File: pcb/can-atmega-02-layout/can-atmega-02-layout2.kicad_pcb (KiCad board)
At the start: 2 copper layers, 114 x 98 mm, 168 parts, among them J1 Screw_Terminal_01x05, J3 Conn_02x03_Odd_Even, J4 Connector_female, U1 LM1117-5.0, U2 TJA1051T, U3 MCP2515-xSO, U4 ATmega328P-A, X1 16MHz, X2 16MHz

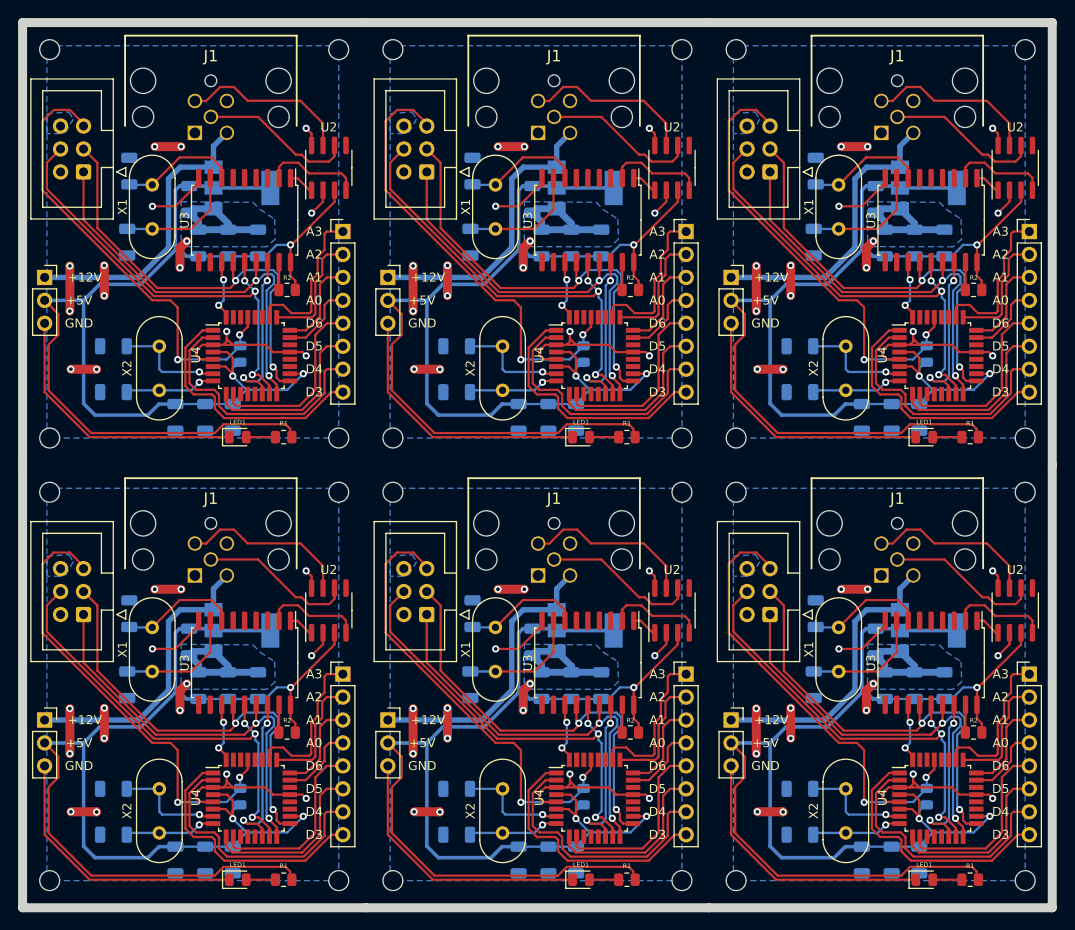
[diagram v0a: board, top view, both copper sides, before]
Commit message: temp-calibrate
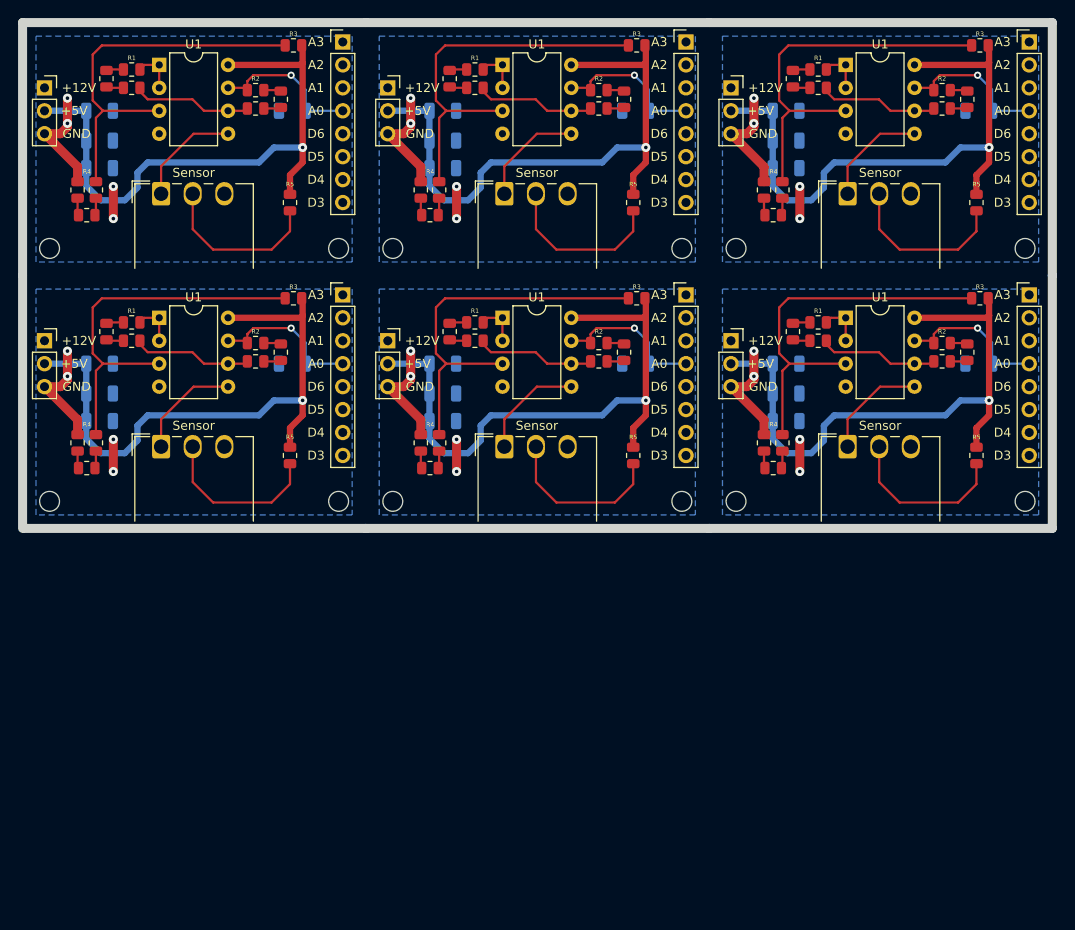
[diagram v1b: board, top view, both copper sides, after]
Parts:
- removed the C1 at (107.9, 33.1)
- removed the C1 at (69.9, 82.1)
- removed the C1 at (69.9, 33.1)
- removed the C1 at (31.9, 82.1)
- removed the C1 at (107.9, 82.1)
- removed the C1 at (31.9, 33.1)
- removed C10 (x6), C11 (x6), C5 (x6), C6 (x6): 22PF, Capacitor_SMD:C_1206_3216Metric
- removed the C2 at (71.0, 37.9)
- removed the C2 at (33.0, 37.9)
- removed the C2 at (109.0, 37.9)
- removed the C2 at (71.0, 86.9)
- removed the C2 at (109.0, 86.9)
- removed the C2 at (33.0, 86.9)
- removed the C3 at (112.3, 37.9)
- removed the C3 at (36.3, 37.9)
- removed the C3 at (112.3, 86.9)
- removed the C3 at (74.3, 37.9)
- removed the C3 at (36.3, 86.9)
- removed the C3 at (74.3, 86.9)
- removed the C4 at (77.6, 37.9)
- removed the C4 at (39.6, 37.9)
- removed the C4 at (39.6, 86.9)
- removed the C4 at (115.6, 86.9)
- removed the C4 at (115.6, 37.9)
- removed the C4 at (77.6, 86.9)
- removed C7 (x6), C9 (x6): 0.1uF, Capacitor_SMD:C_1206_3216Metric
- removed C8 (x6): 10uF/16V, Capacitor_SMD:C_1206_3216Metric
- removed the J1 at (32.6, 74.7)
- removed the J1 at (32.6, 25.7)
- removed the J1 at (70.6, 25.7)
- removed the J1 at (70.6, 74.7)
- removed the J1 at (108.6, 74.7)
- removed the J1 at (108.6, 25.7)
- removed J3 (x6): Conn_02x03_Odd_Even, Connector_IDC:IDC-Header_2x03_P2.54mm_Vertical
- removed J4 (x6): Connector_female, CAN_ATmega:Connector_female
- removed LED1 (x6): Green, LED_SMD:LED_0805_2012Metric
- removed R1 (x6): 1K, Resistor_SMD:R_0805_2012Metric
- removed R2 (x6): 10K, Resistor_SMD:R_0805_2012Metric
- removed the R3 at (75.6, 99.2)
- removed the R3 at (75.6, 50.2)
- removed the R3 at (37.6, 50.2)
- removed the R3 at (37.6, 99.2)
- removed the R3 at (113.6, 99.2)
- removed the R3 at (113.6, 50.2)
- removed the REF** at (48.5, 16.5)
- removed the REF** at (54.5, 59.5)
- removed the REF** at (54.5, 65.5)
- removed the REF** at (86.5, 108.5)
- removed the REF** at (92.5, 65.5)
- removed the REF** at (16.5, 108.5)
- removed the REF** at (16.5, 65.5)
- removed the REF** at (86.5, 16.5)
- removed the REF** at (92.5, 16.5)
- removed the REF** at (48.5, 65.5)
- removed the REF** at (124.5, 16.5)
- removed the REF** at (124.5, 65.5)
- removed the REF** at (124.5, 59.5)
- removed the REF** at (92.5, 59.5)
- removed the REF** at (48.5, 108.5)
- removed the REF** at (124.5, 108.5)
- removed the REF** at (48.5, 59.5)
- removed the REF** at (54.5, 16.5)
- removed the REF** at (92.5, 108.5)
- removed the REF** at (86.5, 65.5)
- removed the REF** at (16.5, 59.5)
- removed the REF** at (16.5, 16.5)
- removed the REF** at (86.5, 59.5)
- removed the REF** at (54.5, 108.5)
- removed the U1 at (75.8, 80.8)
- removed the U1 at (37.8, 31.8)
- removed the U1 at (113.8, 80.8)
- removed the U1 at (75.8, 31.8)
- removed the U1 at (113.8, 31.8)
- removed the U1 at (37.8, 80.8)
- removed U2 (x6): TJA1051T, Package_SO:SOIC-8_3.9x4.9mm_P1.27mm
- removed U3 (x6): MCP2515-xSO, Package_SO:SOIC-18W_7.5x11.6mm_P1.27mm
- removed U4 (x6): ATmega328P-A, Package_QFP:TQFP-32_7x7mm_P0.8mm
- removed X1 (x6), X2 (x6): 16MHz, Crystal:Crystal_HC49-4H_Vertical
- added C1: 100nF, Capacitor_SMD:C_1206_3216Metric, B.Cu at (22.0, 23.3)
- added C1: 100nF, Capacitor_SMD:C_1206_3216Metric, B.Cu at (22.0, 51.3)
- added C1: 100nF, Capacitor_SMD:C_1206_3216Metric, B.Cu at (98.0, 23.3)
- added C1: 100nF, Capacitor_SMD:C_1206_3216Metric, B.Cu at (60.0, 51.3)
- added C1: 100nF, Capacitor_SMD:C_1206_3216Metric, B.Cu at (60.0, 23.3)
- added C1: 100nF, Capacitor_SMD:C_1206_3216Metric, B.Cu at (98.0, 51.3)
- added C2: 100nF, Capacitor_SMD:C_1206_3216Metric, B.Cu at (98.0, 54.6)
- added C2: 100nF, Capacitor_SMD:C_1206_3216Metric, B.Cu at (98.0, 26.6)
- added C2: 100nF, Capacitor_SMD:C_1206_3216Metric, B.Cu at (22.0, 54.6)
- added C2: 100nF, Capacitor_SMD:C_1206_3216Metric, B.Cu at (60.0, 26.6)
- added C2: 100nF, Capacitor_SMD:C_1206_3216Metric, B.Cu at (22.0, 26.6)
- added C2: 100nF, Capacitor_SMD:C_1206_3216Metric, B.Cu at (60.0, 54.6)
- added C3: 10uF/16V, Capacitor_SMD:C_1206_3216Metric, B.Cu at (60.0, 57.6)
- added C3: 10uF/16V, Capacitor_SMD:C_1206_3216Metric, B.Cu at (22.0, 57.6)
- added C3: 10uF/16V, Capacitor_SMD:C_1206_3216Metric, B.Cu at (60.0, 29.6)
- added C3: 10uF/16V, Capacitor_SMD:C_1206_3216Metric, B.Cu at (98.0, 29.6)
- added C3: 10uF/16V, Capacitor_SMD:C_1206_3216Metric, B.Cu at (22.0, 29.6)
- added C3: 10uF/16V, Capacitor_SMD:C_1206_3216Metric, B.Cu at (98.0, 57.6)
- added C4: 100nF, Capacitor_SMD:C_1206_3216Metric, B.Cu at (119.4, 51.3)
- added C4: 100nF, Capacitor_SMD:C_1206_3216Metric, B.Cu at (81.4, 51.3)
- added C4: 100nF, Capacitor_SMD:C_1206_3216Metric, B.Cu at (81.4, 23.3)
- added C4: 100nF, Capacitor_SMD:C_1206_3216Metric, B.Cu at (43.4, 51.3)
- added C4: 100nF, Capacitor_SMD:C_1206_3216Metric, B.Cu at (119.4, 23.3)
- added C4: 100nF, Capacitor_SMD:C_1206_3216Metric, B.Cu at (43.4, 23.3)
- added J1: Connector_male, CAN_ATmega:Connector_male, F.Cu at (107.2, 23.3)
- added J1: Connector_male, CAN_ATmega:Connector_male, F.Cu at (31.2, 51.3)
- added J1: Connector_male, CAN_ATmega:Connector_male, F.Cu at (69.2, 23.3)
- added J1: Connector_male, CAN_ATmega:Connector_male, F.Cu at (107.2, 51.3)
- added J1: Connector_male, CAN_ATmega:Connector_male, F.Cu at (69.2, 51.3)
- added J1: Connector_male, CAN_ATmega:Connector_male, F.Cu at (31.2, 23.3)
- added J2: Screw_Terminal_01x03, Connector_Wago:Wago_734-163_1x03_P3.50mm_Horizontal, F.Cu at (66.8, 32.5)
- added J2: Screw_Terminal_01x03, Connector_Wago:Wago_734-163_1x03_P3.50mm_Horizontal, F.Cu at (28.8, 32.5)
- added J2: Screw_Terminal_01x03, Connector_Wago:Wago_734-163_1x03_P3.50mm_Horizontal, F.Cu at (104.8, 60.5)
- added J2: Screw_Terminal_01x03, Connector_Wago:Wago_734-163_1x03_P3.50mm_Horizontal, F.Cu at (66.8, 60.5)
- added J2: Screw_Terminal_01x03, Connector_Wago:Wago_734-163_1x03_P3.50mm_Horizontal, F.Cu at (104.8, 32.5)
- added J2: Screw_Terminal_01x03, Connector_Wago:Wago_734-163_1x03_P3.50mm_Horizontal, F.Cu at (28.8, 60.5)
- added R1_1: 1.3k, Resistor_SMD:R_0805_2012Metric, F.Cu at (101.6, 18.7)
- added R1_1: 1.3k, Resistor_SMD:R_0805_2012Metric, F.Cu at (101.6, 46.7)
- added R1_1: 1.3k, Resistor_SMD:R_0805_2012Metric, F.Cu at (63.6, 46.7)
- added R1_1: 1.3k, Resistor_SMD:R_0805_2012Metric, F.Cu at (25.6, 46.7)
- added R1_1: 1.3k, Resistor_SMD:R_0805_2012Metric, F.Cu at (25.6, 18.7)
- added R1_1: 1.3k, Resistor_SMD:R_0805_2012Metric, F.Cu at (63.6, 18.7)
- added R1_2: 2k, Resistor_SMD:R_0805_2012Metric, F.Cu at (60.8, 47.7)
- added R1_2: 2k, Resistor_SMD:R_0805_2012Metric, F.Cu at (22.8, 47.7)
- added R1_2: 2k, Resistor_SMD:R_0805_2012Metric, F.Cu at (22.8, 19.7)
- added R1_2: 2k, Resistor_SMD:R_0805_2012Metric, F.Cu at (98.8, 47.7)
- added R1_2: 2k, Resistor_SMD:R_0805_2012Metric, F.Cu at (98.8, 19.7)
- added R1_2: 2k, Resistor_SMD:R_0805_2012Metric, F.Cu at (60.8, 19.7)
- added R1_3: 10k, Resistor_SMD:R_0805_2012Metric, F.Cu at (63.6, 20.7)
- added R1_3: 10k, Resistor_SMD:R_0805_2012Metric, F.Cu at (101.6, 48.7)
- added R1_3: 10k, Resistor_SMD:R_0805_2012Metric, F.Cu at (25.6, 20.7)
- added R1_3: 10k, Resistor_SMD:R_0805_2012Metric, F.Cu at (101.6, 20.7)
- added R1_3: 10k, Resistor_SMD:R_0805_2012Metric, F.Cu at (63.6, 48.7)
- added R1_3: 10k, Resistor_SMD:R_0805_2012Metric, F.Cu at (25.6, 48.7)
- added R2_1: 330, Resistor_SMD:R_0805_2012Metric, F.Cu at (115.3, 23.0)
- added R2_1: 330, Resistor_SMD:R_0805_2012Metric, F.Cu at (77.3, 23.0)
- added R2_1: 330, Resistor_SMD:R_0805_2012Metric, F.Cu at (39.3, 23.0)
- added R2_1: 330, Resistor_SMD:R_0805_2012Metric, F.Cu at (115.3, 51.0)
- added R2_1: 330, Resistor_SMD:R_0805_2012Metric, F.Cu at (39.3, 51.0)
- added R2_1: 330, Resistor_SMD:R_0805_2012Metric, F.Cu at (77.3, 51.0)
- added R2_2: 1.3k, Resistor_SMD:R_0805_2012Metric, F.Cu at (42.1, 22.0)
- added R2_2: 1.3k, Resistor_SMD:R_0805_2012Metric, F.Cu at (80.1, 22.0)
- added R2_2: 1.3k, Resistor_SMD:R_0805_2012Metric, F.Cu at (118.1, 22.0)
- added R2_2: 1.3k, Resistor_SMD:R_0805_2012Metric, F.Cu at (80.1, 50.0)
- added R2_2: 1.3k, Resistor_SMD:R_0805_2012Metric, F.Cu at (118.1, 50.0)
- added R2_2: 1.3k, Resistor_SMD:R_0805_2012Metric, F.Cu at (42.1, 50.0)
- added R2_3: 110k, Resistor_SMD:R_0805_2012Metric, F.Cu at (77.3, 21.0)
- added R2_3: 110k, Resistor_SMD:R_0805_2012Metric, F.Cu at (39.3, 21.0)
- added R2_3: 110k, Resistor_SMD:R_0805_2012Metric, F.Cu at (39.3, 49.0)
- added R2_3: 110k, Resistor_SMD:R_0805_2012Metric, F.Cu at (77.3, 49.0)
- added R2_3: 110k, Resistor_SMD:R_0805_2012Metric, F.Cu at (115.3, 21.0)
- added R2_3: 110k, Resistor_SMD:R_0805_2012Metric, F.Cu at (115.3, 49.0)
- added R3: 20k, Resistor_SMD:R_0805_2012Metric, F.Cu at (81.5, 44.0)
- added R3: 20k, Resistor_SMD:R_0805_2012Metric, F.Cu at (119.5, 16.0)
- added R3: 20k, Resistor_SMD:R_0805_2012Metric, F.Cu at (43.5, 16.0)
- added R3: 20k, Resistor_SMD:R_0805_2012Metric, F.Cu at (81.5, 16.0)
- added R3: 20k, Resistor_SMD:R_0805_2012Metric, F.Cu at (119.5, 44.0)
- added R3: 20k, Resistor_SMD:R_0805_2012Metric, F.Cu at (43.5, 44.0)
- added R4_1: 2k, Resistor_SMD:R_0805_2012Metric, F.Cu at (57.6, 32.0)
- added R4_1: 2k, Resistor_SMD:R_0805_2012Metric, F.Cu at (19.6, 32.0)
- added R4_1: 2k, Resistor_SMD:R_0805_2012Metric, F.Cu at (95.6, 60.0)
- added R4_1: 2k, Resistor_SMD:R_0805_2012Metric, F.Cu at (57.6, 60.0)
- added R4_1: 2k, Resistor_SMD:R_0805_2012Metric, F.Cu at (95.6, 32.0)
- added R4_1: 2k, Resistor_SMD:R_0805_2012Metric, F.Cu at (19.6, 60.0)
- added R4_2: 2.4k, Resistor_SMD:R_0805_2012Metric, F.Cu at (20.6, 34.8)
- added R4_2: 2.4k, Resistor_SMD:R_0805_2012Metric, F.Cu at (96.6, 62.8)
- added R4_2: 2.4k, Resistor_SMD:R_0805_2012Metric, F.Cu at (58.6, 34.8)
- added R4_2: 2.4k, Resistor_SMD:R_0805_2012Metric, F.Cu at (20.6, 62.8)
- added R4_2: 2.4k, Resistor_SMD:R_0805_2012Metric, F.Cu at (58.6, 62.8)
- added R4_2: 2.4k, Resistor_SMD:R_0805_2012Metric, F.Cu at (96.6, 34.8)
- added R4_3: 20k, Resistor_SMD:R_0805_2012Metric, F.Cu at (97.6, 32.0)
- added R4_3: 20k, Resistor_SMD:R_0805_2012Metric, F.Cu at (21.6, 60.0)
- added R4_3: 20k, Resistor_SMD:R_0805_2012Metric, F.Cu at (59.6, 32.0)
- added R4_3: 20k, Resistor_SMD:R_0805_2012Metric, F.Cu at (21.6, 32.0)
- added R4_3: 20k, Resistor_SMD:R_0805_2012Metric, F.Cu at (97.6, 60.0)
- added R4_3: 20k, Resistor_SMD:R_0805_2012Metric, F.Cu at (59.6, 60.0)
- added R5: 1k, Resistor_SMD:R_0805_2012Metric, F.Cu at (43.1, 33.4)
- added R5: 1k, Resistor_SMD:R_0805_2012Metric, F.Cu at (119.1, 61.4)
- added R5: 1k, Resistor_SMD:R_0805_2012Metric, F.Cu at (119.1, 33.4)
- added R5: 1k, Resistor_SMD:R_0805_2012Metric, F.Cu at (81.1, 33.4)
- added R5: 1k, Resistor_SMD:R_0805_2012Metric, F.Cu at (43.1, 61.4)
- added R5: 1k, Resistor_SMD:R_0805_2012Metric, F.Cu at (81.1, 61.4)
- added REF**: MountingHole_2.2mm_M2, MountingHole:MountingHole_2.2mm_M2, F.Cu at (92.5, 66.5)
- added REF**: MountingHole_2.2mm_M2, MountingHole:MountingHole_2.2mm_M2, F.Cu at (124.5, 38.5)
- added REF**: MountingHole_2.2mm_M2, MountingHole:MountingHole_2.2mm_M2, F.Cu at (54.5, 66.5)
- added REF**: MountingHole_2.2mm_M2, MountingHole:MountingHole_2.2mm_M2, F.Cu at (92.5, 38.5)
- added REF**: MountingHole_2.2mm_M2, MountingHole:MountingHole_2.2mm_M2, F.Cu at (16.5, 66.5)
- added REF**: MountingHole_2.2mm_M2, MountingHole:MountingHole_2.2mm_M2, F.Cu at (54.5, 38.5)
- added REF**: MountingHole_2.2mm_M2, MountingHole:MountingHole_2.2mm_M2, F.Cu at (48.5, 38.5)
- added REF**: MountingHole_2.2mm_M2, MountingHole:MountingHole_2.2mm_M2, F.Cu at (86.5, 38.5)
- added REF**: MountingHole_2.2mm_M2, MountingHole:MountingHole_2.2mm_M2, F.Cu at (86.5, 66.5)
- added REF**: MountingHole_2.2mm_M2, MountingHole:MountingHole_2.2mm_M2, F.Cu at (16.5, 38.5)
- added REF**: MountingHole_2.2mm_M2, MountingHole:MountingHole_2.2mm_M2, F.Cu at (124.5, 66.5)
- added REF**: MountingHole_2.2mm_M2, MountingHole:MountingHole_2.2mm_M2, F.Cu at (48.5, 66.5)
- added U1: MCP6002-xP, Package_DIP:DIP-8_W7.62mm, F.Cu at (28.6, 46.2)
- added U1: MCP6002-xP, Package_DIP:DIP-8_W7.62mm, F.Cu at (104.6, 18.2)
- added U1: MCP6002-xP, Package_DIP:DIP-8_W7.62mm, F.Cu at (66.6, 18.2)
- added U1: MCP6002-xP, Package_DIP:DIP-8_W7.62mm, F.Cu at (66.6, 46.2)
- added U1: MCP6002-xP, Package_DIP:DIP-8_W7.62mm, F.Cu at (28.6, 18.2)
- added U1: MCP6002-xP, Package_DIP:DIP-8_W7.62mm, F.Cu at (104.6, 46.2)
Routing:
- net +5V: track 922.4 -> 398.4 mm, vias 18 -> 6
- net GND: track 554.3 -> 98.5 mm, vias 90 -> 24
- net U4_RST: track 305.2 -> 0.00 mm, vias 12 -> 0
- net U4_D11_MOSI: track 300.0 -> 0.00 mm, vias 18 -> 0
- net U4_D13_SCK: track 295.2 -> 0.00 mm, vias 12 -> 0
- net U4_D12_MISO: track 279.1 -> 0.00 mm, vias 12 -> 0
- net /vk_in: track 0.00 -> 257.0 mm
- net +12V: track 195.7 -> 0.00 mm
- net U4_D4: track 176.6 -> 0.00 mm
- net U4_D3: track 173.6 -> 0.00 mm
- net U4_D6: track 123.8 -> 0.00 mm
- net U4_D5: track 118.3 -> 0.00 mm
- net CAN_H: track 113.7 -> 0.00 mm
- net /S2: track 0.00 -> 112.4 mm
- net D10_CS: track 112.4 -> 0.00 mm, vias 12 -> 0
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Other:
- board size 114 x 98 mm -> 114 x 56 mm
- board text added: "GND"
- board text added: "R1"
- board text added: "R2"
- board text added: "R4"
- board text added: "Sensor"
